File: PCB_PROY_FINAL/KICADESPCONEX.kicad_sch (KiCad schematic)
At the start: 16 parts, among them IC2 ESP32-S3-WROOM-1-N16, SW1 SW_Push

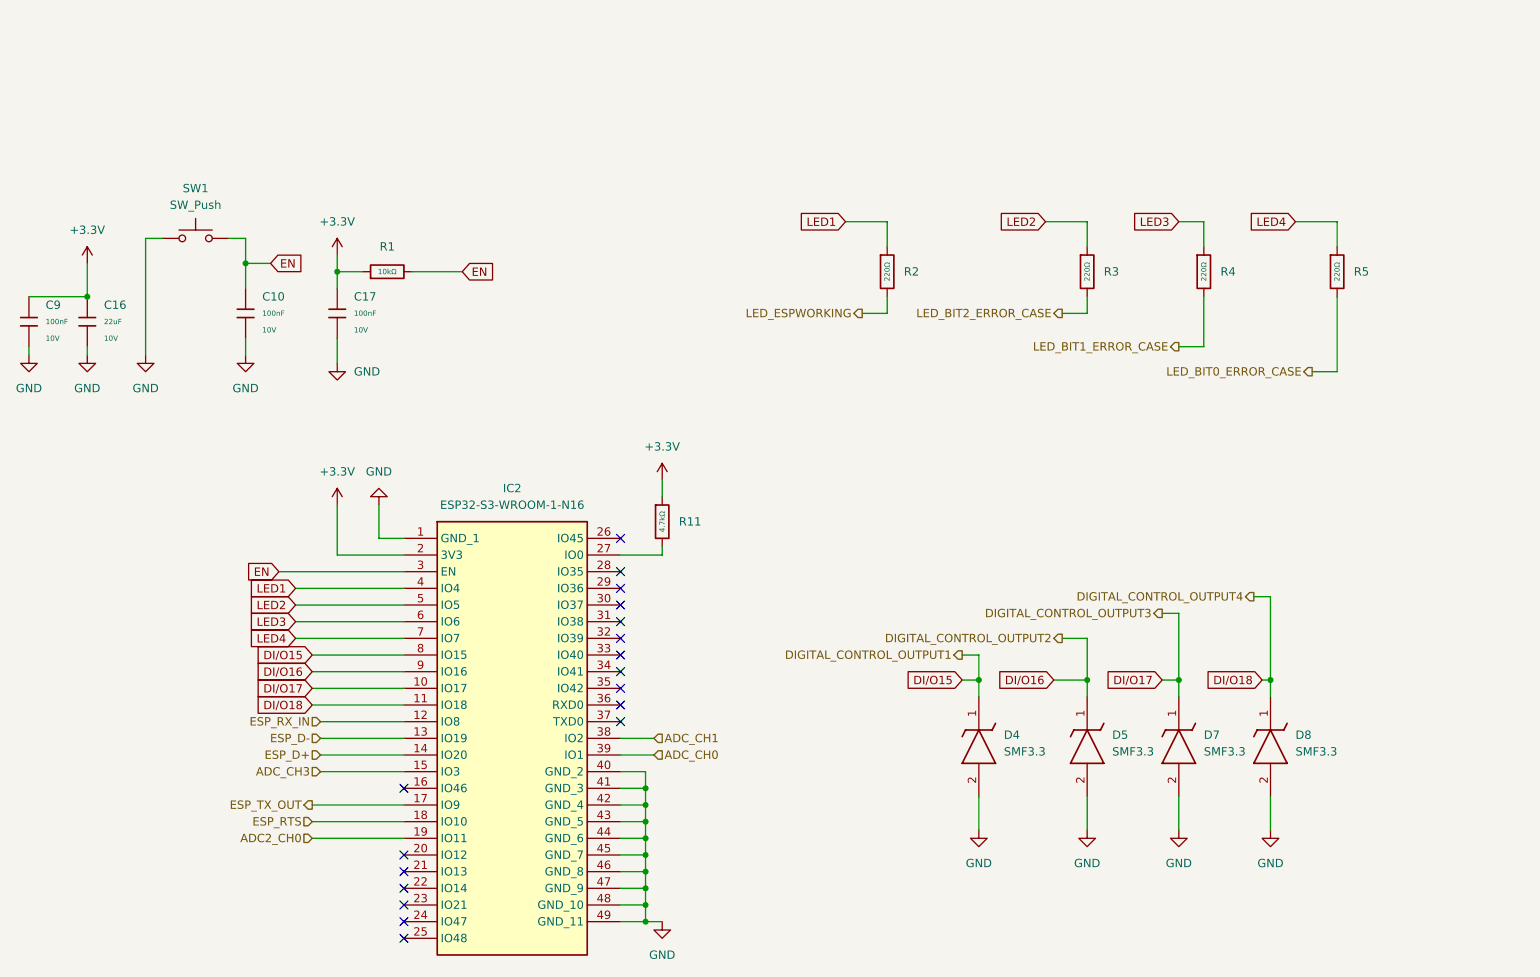
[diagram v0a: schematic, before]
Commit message: Update
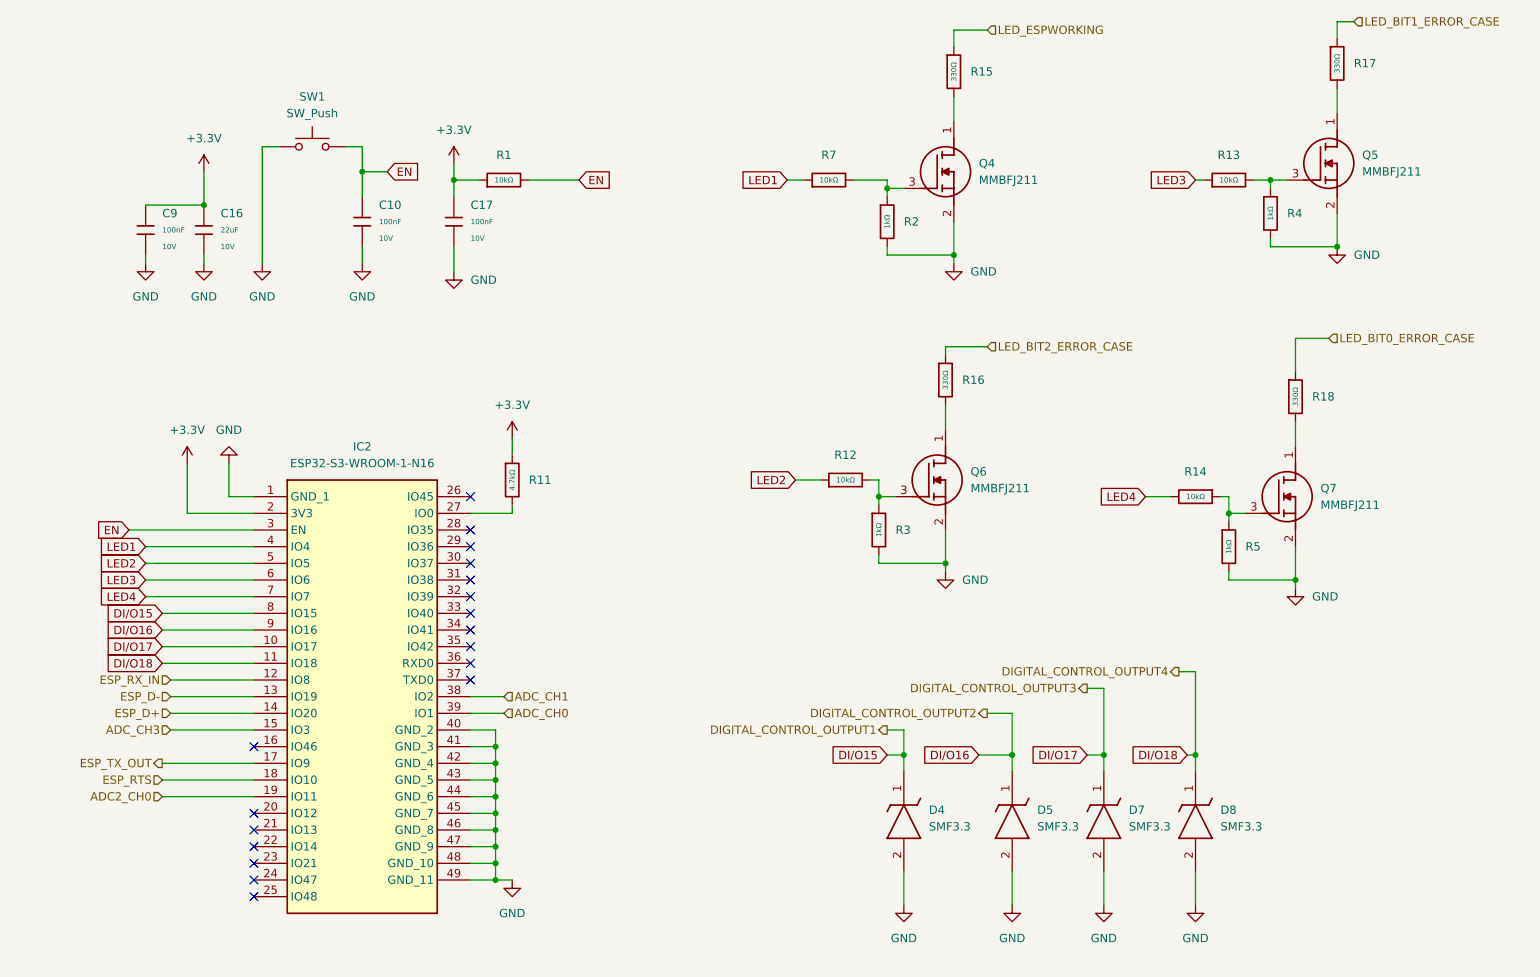
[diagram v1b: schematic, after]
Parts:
- removed R2, R3, R4, R5: 220Ω, PCM_JLCPCB:R_0603, symbol PCM_JLCPCB-Resistors:0603,220Ω
- added Q4, Q5, Q6, Q7: MMBFJ211, SOT95P251X112-3N, symbol SamacSys_Parts:MMBFJ211
- added R12, R13, R14, R7: 10kΩ, PCM_JLCPCB:R_1206, symbol PCM_JLCPCB-Resistors:1206,10kΩ
- added R15, R16, R17, R18: 330Ω, PCM_JLCPCB:R_1206, symbol PCM_JLCPCB-Resistors:1206,330Ω
- added R2, R3, R4, R5: 1kΩ, PCM_JLCPCB:R_1206, symbol PCM_JLCPCB-Resistors:1206,1kΩ
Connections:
- net GND: now also Q4.2 (S), Q5.2 (S), Q6.2 (S), Q7.2 (S), R2.2, R3.2, R4.2, R5.2
- net LED1: now also R7.1
- net LED2: now also R12.1
- net LED3: now also R13.1
- net LED4: now also R14.2
- net LED_BIT0_ERROR_CASE: now also R18.1
- net LED_BIT1_ERROR_CASE: now also R17.1
- net LED_BIT2_ERROR_CASE: now also R16.1
- net LED_ESPWORKING: now also R15.1
- new net: Q5.1 (D), R17.2
- new net: Q5.3 (G), R13.2, R4.1
- new net: Q4.3 (G), R2.1, R7.2
- new net: Q6.3 (G), R12.2, R3.1
- new net: Q7.3 (G), R14.1, R5.1
- new net: Q4.1 (D), R15.2
- new net: Q7.1 (D), R18.2
- new net: Q6.1 (D), R16.2
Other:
- moved on the sheet: C10, C16, C17, C9, D4, D5, D7, D8, IC2, R1, R11, SW1
